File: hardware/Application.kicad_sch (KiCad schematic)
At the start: 1 part, among them U101 STM32G431C6Ux

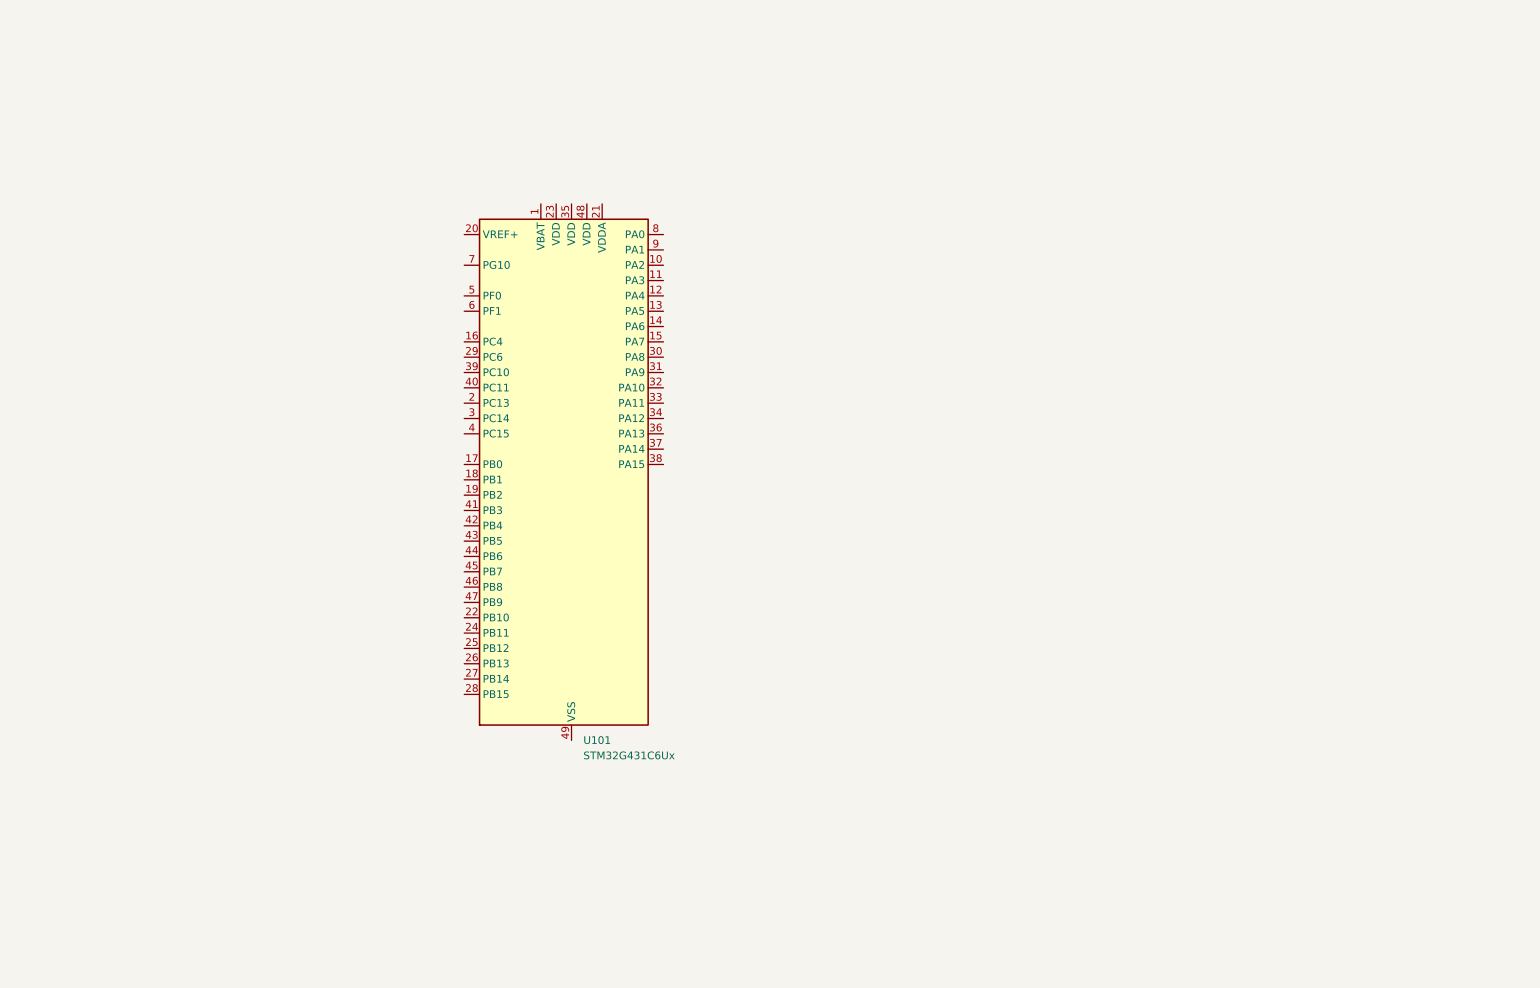
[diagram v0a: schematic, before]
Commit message: asdf
Signed-off-by: Connor Rigby <connorr@hey.com>
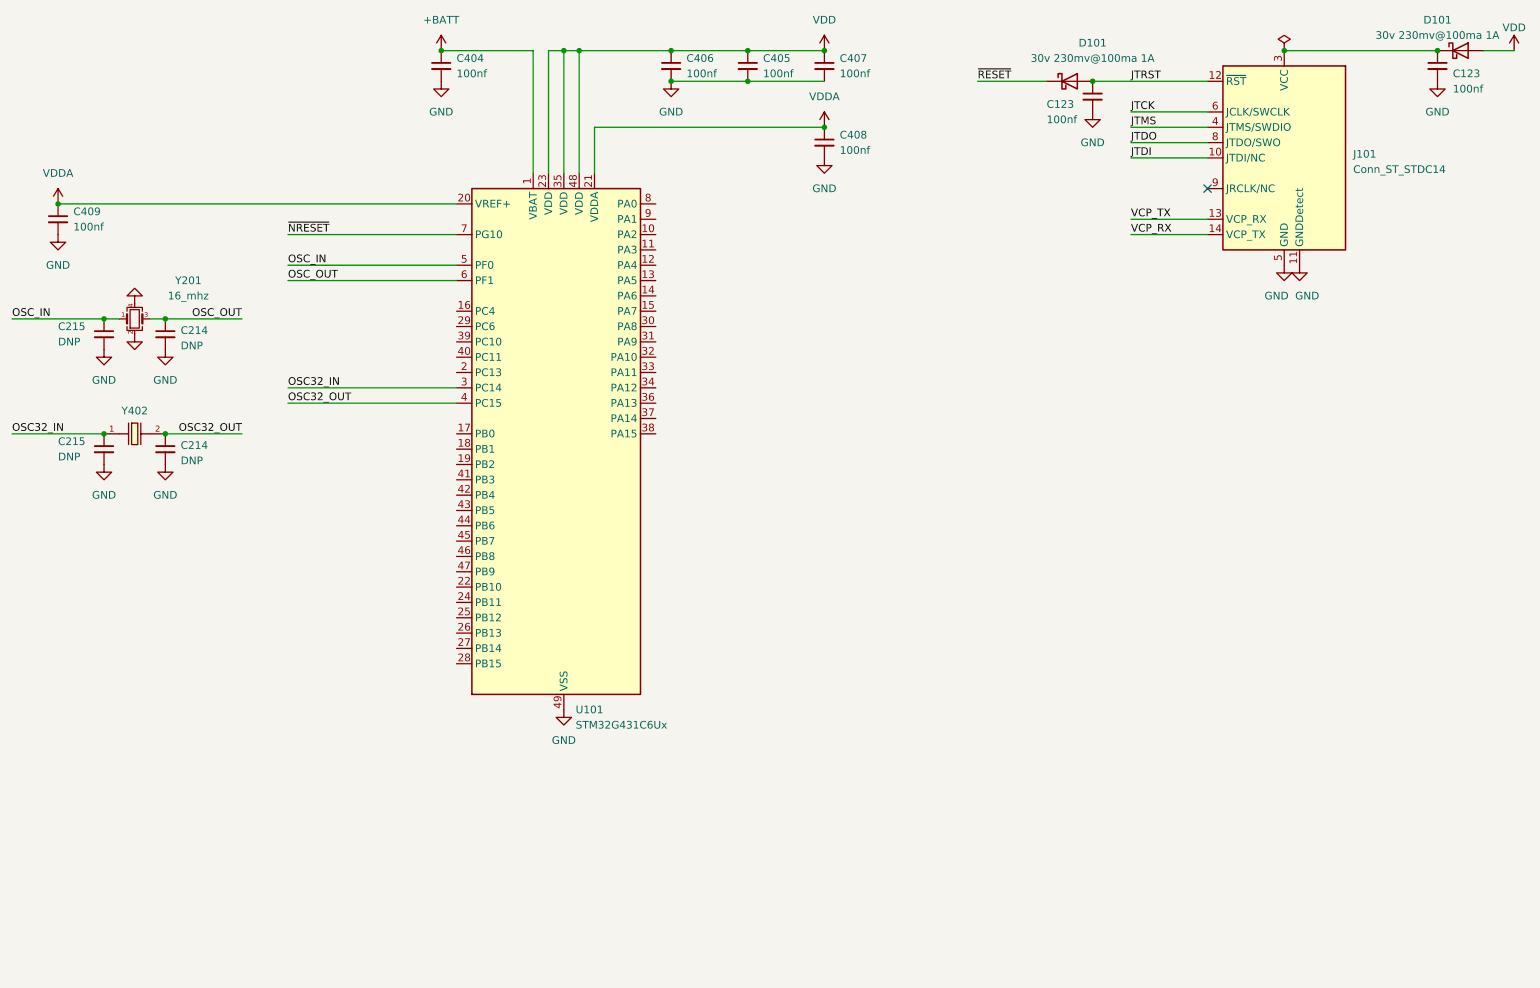
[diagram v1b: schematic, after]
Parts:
- added C123 (x2), C404, C405, C406, C407, C408, C409: C_0402_100nf_X7R, Capacitor_SMD:C_0402_1005Metric, symbol LCSC_Capacitor:C_0402_100nf_X7R
- added C214 (x2), C215 (x2): C_0402_DNP, Capacitor_SMD:C_0402_1005Metric, symbol LCSC_Capacitor:C_0402_DNP
- added D101 (x2): 30v 230mv@100ma 1A, Diode_SMD:D_SOD-323F, symbol Device:D_Schottky
- added J101: Conn_ST_STDC14, LCSC_Connector:TC2070-IDC-FP, symbol Connector:Conn_ST_STDC14
- added Y201: 16_mhz, Crystal:Crystal_SMD_3225-4Pin_3.2x2.5mm, symbol LCSC_Crystal:Crystal_GND24_DNP
- added Y402: Q13FC1350000400, Crystal:Crystal_SMD_3215-2Pin_3.2x1.5mm, symbol LCSC_Crystal:Q13FC1350000400
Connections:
- net +BATT: now reaches U101.1 (VBAT)
- net +BATT: now also C404.1
- net VDDA: now reaches U101.20 (VREF+)
- net VDDA: now also U101.21 (VDDA), C408.1, C409.1
- net VDD: now reaches U101.23 (VDD)
- net VDD: now also U101.35 (VDD), U101.48 (VDD), C405.1, C406.1, C407.1, D101.2 (A)
- net OSC32_IN: now reaches U101.3 (PC14)
- net OSC32_IN: now also C215.1, Y402.1
- net OSC32_OUT: now reaches U101.4 (PC15)
- net OSC32_OUT: now also C214.1, Y402.2
- net GND: now reaches U101.49 (VSS)
- net GND: now also C123.2, C123.2, C214.2, C214.2, C215.2, C215.2, C404.2, C405.2, C406.2, C407.2, C408.2, C409.2, J101.11 (GNDDetect), J101.5 (GND), J101.7 (GND), Y201.2, Y201.4
- net OSC_IN: now reaches U101.5 (PF0)
- net OSC_IN: now also C215.1, Y201.1
- net OSC_OUT: now reaches U101.6 (PF1)
- net OSC_OUT: now also C214.1, Y201.3
- net ~{NRESET}: now reaches U101.7 (PG10)
- new net: C123.1, D101.1 (K), J101.3 (VCC)
- new net JTCK: J101.6 (JCLK/SWCLK)
- new net JTDI: J101.10 (JTDI/NC)
- new net JTDO: J101.8 (JTDO/SWO)
- new net JTMS: J101.4 (JTMS/SWDIO)
- new net JTRST: C123.1, D101.2 (A), J101.12 (~{RST})
- new net VCP_RX: J101.14 (VCP_TX)
- new net VCP_TX: J101.13 (VCP_RX)
- new net ~{RESET}: D101.1 (K)
- no-connect marks 0 -> 1
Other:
- moved on the sheet: U101

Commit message: asdf
Signed-off-by: Connor Rigby <connorr@hey.com>
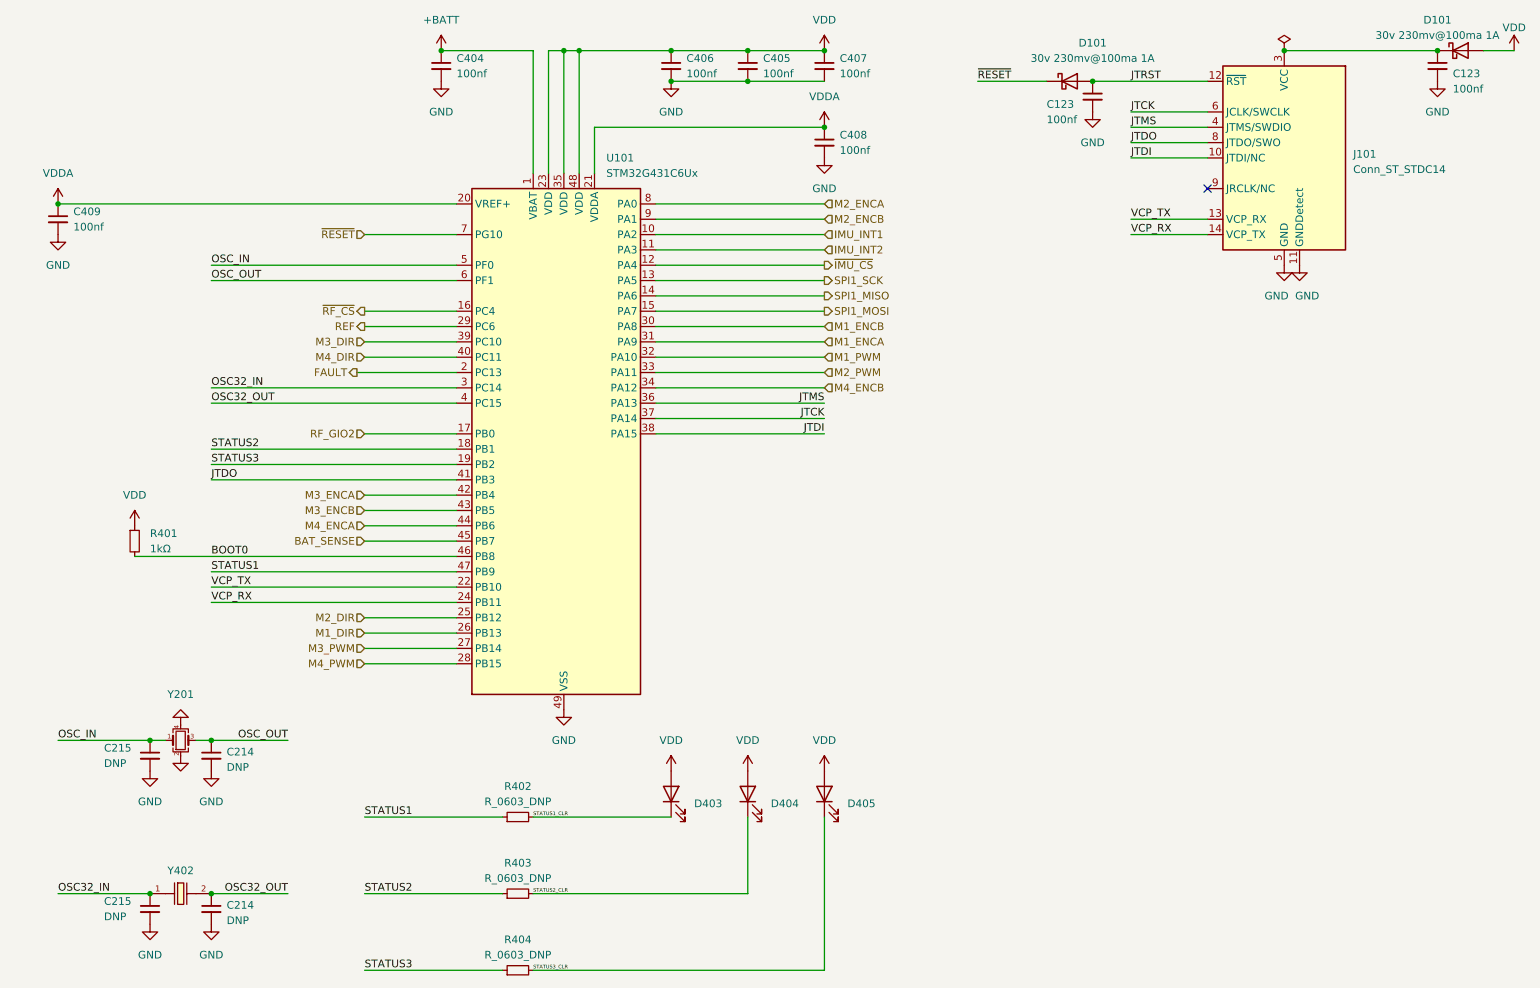
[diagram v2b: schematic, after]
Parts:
- added D403, D404, D405: LED_0603_DNP, LED_SMD:LED_0603_1608Metric, symbol LCSC_LED:LED_0603_DNP
- added R401: R_0402_1k, Resistor_SMD:R_0402_1005Metric, symbol LCSC_Resistor:R_0402_1k
- added R402, R403, R404: R_0603_DNP, Resistor_SMD:R_0603_1608Metric, symbol LCSC_Resistor:R_0603_DNP
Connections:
- net ~{NRESET} is gone; now on net ~{RESET}: U101.7 (PG10)
- net JTCK: now also U101.37 (PA14)
- net JTDI: now also U101.38 (PA15)
- net JTDO: now also U101.41 (PB3)
- net JTMS: now also U101.36 (PA13)
- net VCP_RX: now also U101.24 (PB11)
- net VCP_TX: now also U101.22 (PB10)
- net VDD: now also D403.2 (A), D404.2 (A), D405.2 (A), R401.1
- net IMU_INT1: now reaches U101.10 (PA2)
- net IMU_INT2: now reaches U101.11 (PA3)
- net ~{IMU_CS}: now reaches U101.12 (PA4)
- net SPI1_SCK: now reaches U101.13 (PA5)
- net SPI1_MISO: now reaches U101.14 (PA6)
- net SPI1_MOSI: now reaches U101.15 (PA7)
- net ~{RF_CS}: now reaches U101.16 (PC4)
- net RF_GIO2: now reaches U101.17 (PB0)
- net STATUS2: now reaches U101.18 (PB1)
- net STATUS2: now also R403.1
- net STATUS3: now reaches U101.19 (PB2)
- net STATUS3: now also R404.1
- net FAULT: now reaches U101.2 (PC13)
- net M2_DIR: now reaches U101.25 (PB12)
- net M1_DIR: now reaches U101.26 (PB13)
- net M3_PWM: now reaches U101.27 (PB14)
- net M4_PWM: now reaches U101.28 (PB15)
- net REF: now reaches U101.29 (PC6)
- net M1_ENCB: now reaches U101.30 (PA8)
- net M1_ENCA: now reaches U101.31 (PA9)
- net M1_PWM: now reaches U101.32 (PA10)
- net M2_PWM: now reaches U101.33 (PA11)
- net M4_ENCB: now reaches U101.34 (PA12)
- net M3_DIR: now reaches U101.39 (PC10)
- net M4_DIR: now reaches U101.40 (PC11)
- net M3_ENCA: now reaches U101.42 (PB4)
- net M3_ENCB: now reaches U101.43 (PB5)
- net M4_ENCA: now reaches U101.44 (PB6)
- net BAT_SENSE: now reaches U101.45 (PB7)
- net BOOT0: now reaches U101.46 (PB8)
- net BOOT0: now also R401.2
- net STATUS1: now reaches U101.47 (PB9)
- net STATUS1: now also R402.1
- net M2_ENCA: now reaches U101.8 (PA0)
- net M2_ENCB: now reaches U101.9 (PA1)
- new net STATUS1_CLR: D403.1 (K), R402.2
- new net STATUS2_CLR: D404.1 (K), R403.2
- new net STATUS3_CLR: D405.1 (K), R404.2
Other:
- moved on the sheet: C214, C215, Y201, Y402
